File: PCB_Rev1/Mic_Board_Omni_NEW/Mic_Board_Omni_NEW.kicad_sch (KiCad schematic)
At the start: 31 parts, among them J2 532610771, J3 S2B-ZR-SM4A-TF_LF__SN_, U1 OPA1671IDBVR

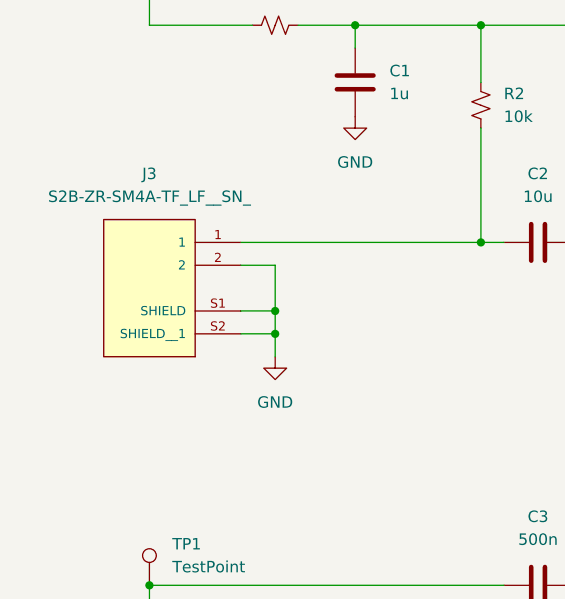
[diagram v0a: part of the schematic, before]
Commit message: MICBOARD OMNI CSV DONE
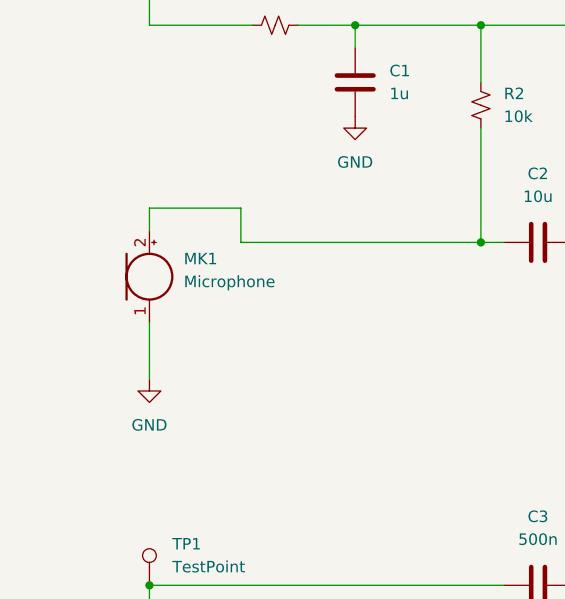
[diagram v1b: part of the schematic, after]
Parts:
- removed J3: S2B-ZR-SM4A-TF_LF__SN_, Footprints:Mic_Conn, symbol Mic Connectors:S2B-ZR-SM4A-TF_LF__SN_
- added MK1: Microphone, Footprints:Omnidirectional, symbol Device:Microphone
- C1, C10, C8, C9: LCSC (none) -> C519973
- C11: LCSC (none) -> C519977
- C2, C5, C6, C7: LCSC (none) -> C88484
- C3: LCSC (none) -> C576434
- C4: LCSC (none) -> C3857194
- J2: LCSC (none) -> C505276
- R1: LCSC (none) -> C865529
- R2, R8, R9: LCSC (none) -> C110775
- R3, R4: LCSC (none) -> C96346
- R5: LCSC (none) -> C95781
- R6: LCSC (none) -> C868262
- R7: LCSC (none) -> C137468
- U1: LCSC (none) -> C1849409
- U2: LCSC (none) -> C1519002
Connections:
- net GND: now also MK1.1 (-)
- net at C2.1, R2.2: now also MK1.2 (+)
